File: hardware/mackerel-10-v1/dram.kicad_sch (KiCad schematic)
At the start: 30 parts, among them J2 Conn_02x05_Odd_Even

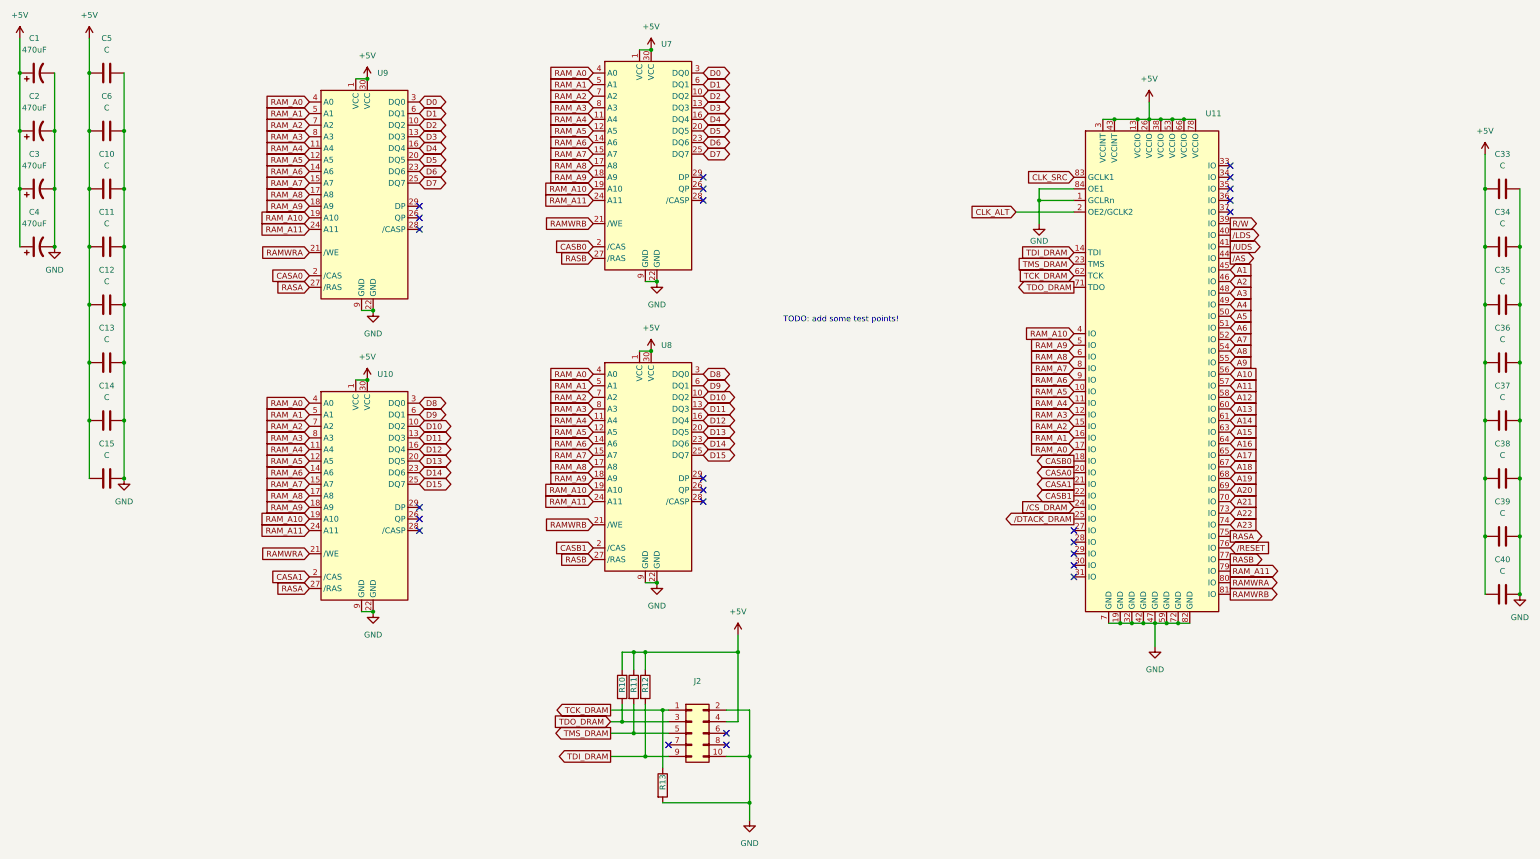
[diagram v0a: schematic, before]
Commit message: Mackerel-10 v1 release
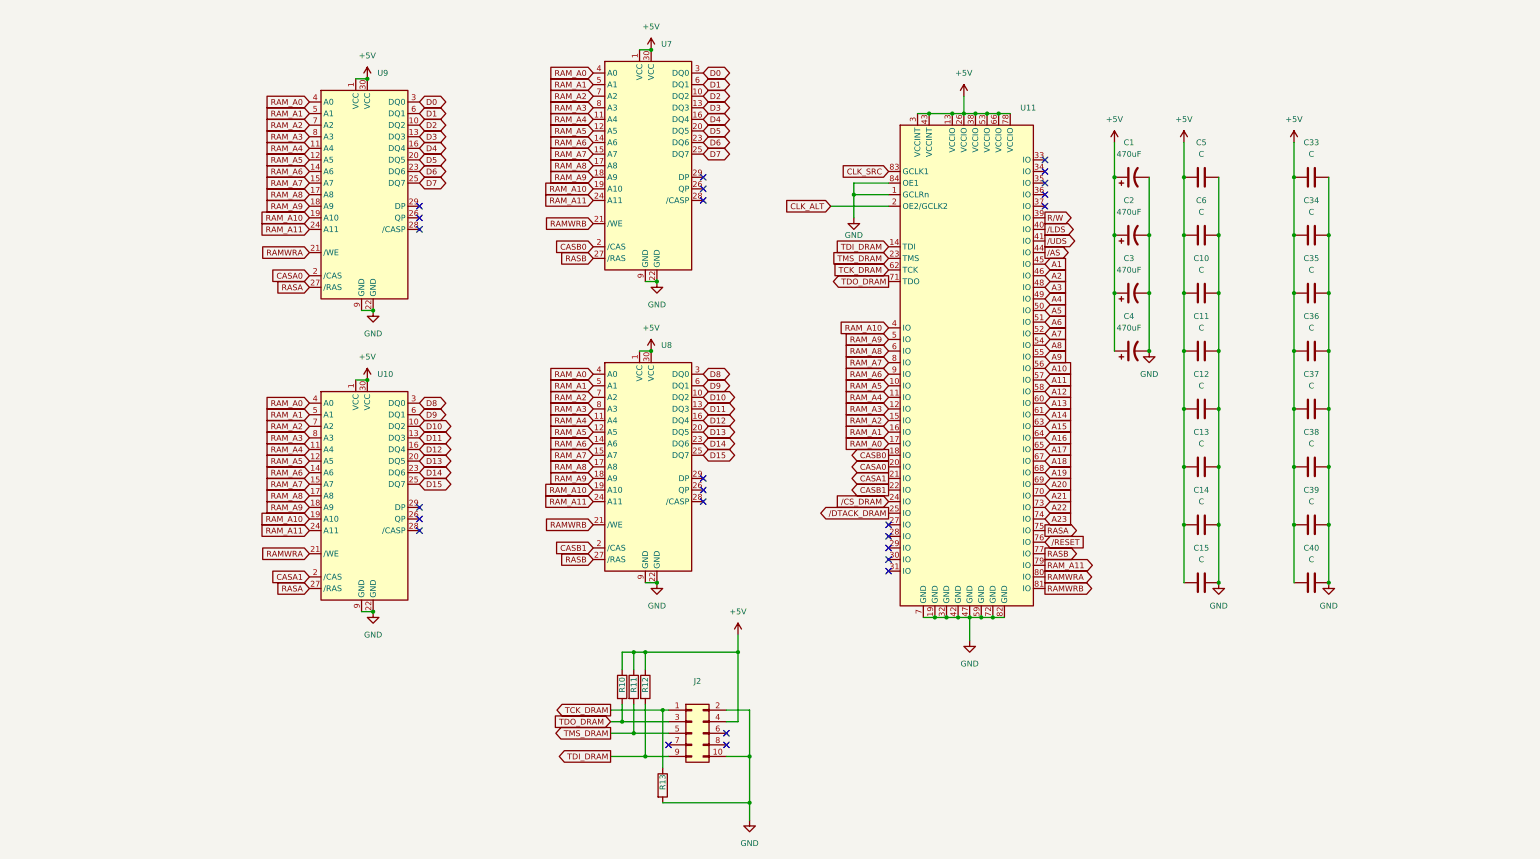
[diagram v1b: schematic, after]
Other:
- note removed: "TODO: add some test points!"
- moved on the sheet: C1, C10, C11, C12, C13, C14, C15, C2, C3, C33, C34, C35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
